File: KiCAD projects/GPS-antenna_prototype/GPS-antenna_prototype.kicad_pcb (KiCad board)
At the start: 2 copper layers, 71.1 x 134.6 mm, 1 part, among them J1 MMCX_Connector

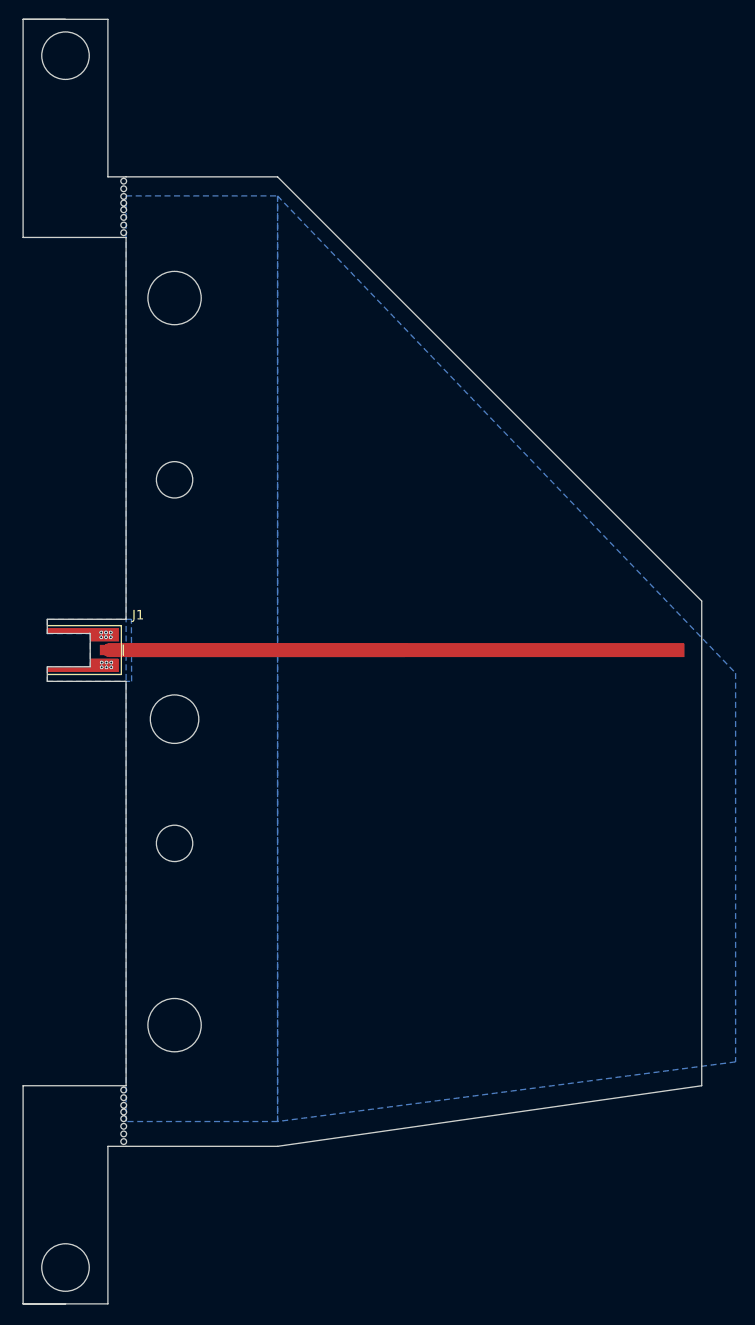
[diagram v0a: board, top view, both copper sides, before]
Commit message: finished creating production files
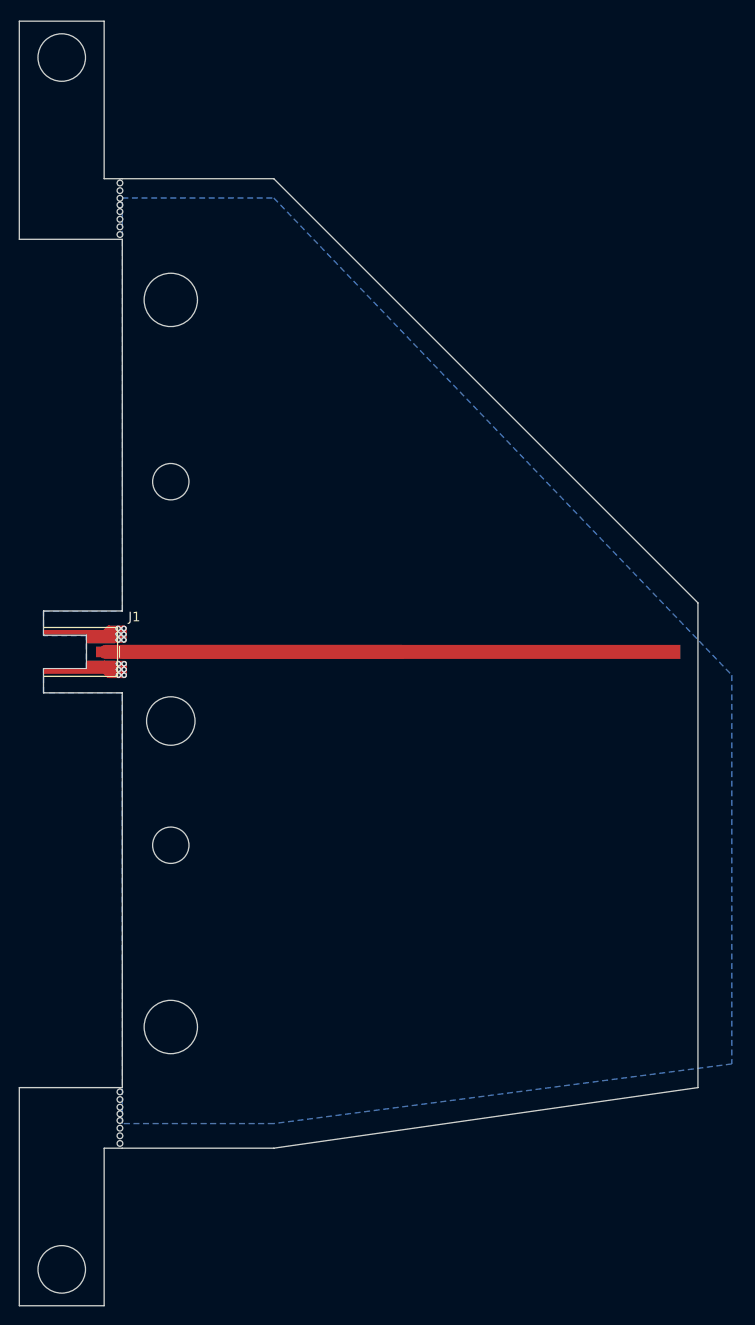
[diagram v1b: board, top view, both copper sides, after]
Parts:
- moved J1 0.44 mm to (80.0, 100.8)
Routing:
- net GroundPlane: track 0.00 -> 21.5 mm
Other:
- outline, holes or cut-outs redrawn
